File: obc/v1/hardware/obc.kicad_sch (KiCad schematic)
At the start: 41 parts, among them J4 USB_C_Receptacle_USB2.0_16P, U10 LM66100DCK, U11 LM66100DCK, U12 USBLC6-2P6, U9 AMS1117-3.3

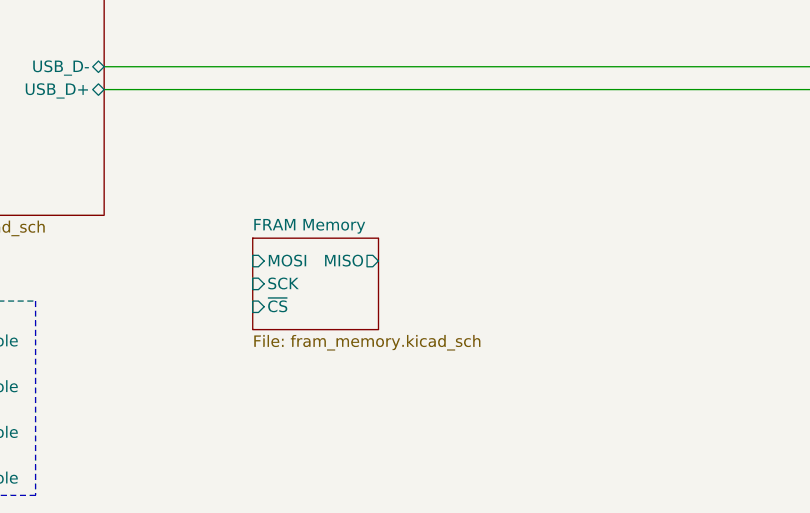
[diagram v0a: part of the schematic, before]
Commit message: fixes
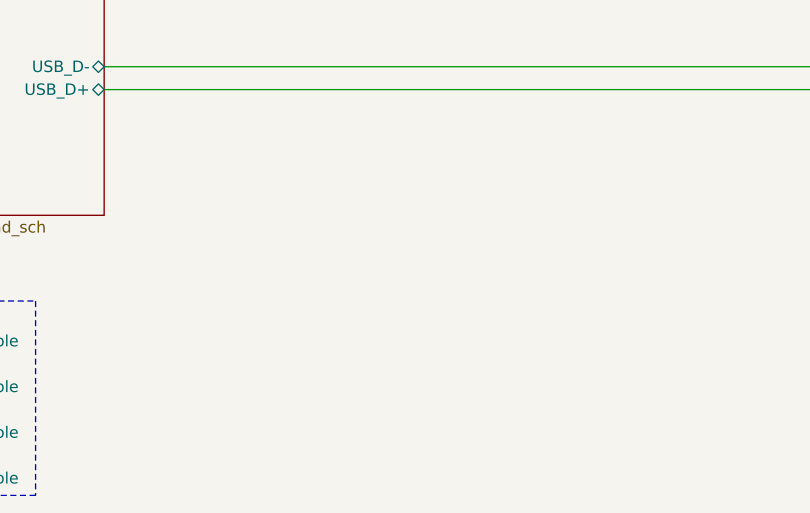
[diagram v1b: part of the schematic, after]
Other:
- removed sheet FRAM Memory
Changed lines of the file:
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@@
-	)
-	(sheet
-		(at 63.5 151.13)
-		(size 13.97 10.16)
-		(exclude_from_sim no)
-		(in_bom yes)
-		(on_board yes)
-		(dnp no)
-		(fields_autoplaced yes)
-		(stroke
-			(width 0.1524)
-			(type solid)
-		)
-		(fill
-			(color 0 0 0 0)
-		)
-		(property "Sheetname" "FRAM Memory"
-			(at 63.5 150.4184 0)
-			(show_name no)
-			(do_not_autoplace no)
-			(effects
-				(font
-					(size 1.27 1.27)
-				)
-				(justify left bottom)
-			)
-		)
-		(property "Sheetfile" "fram_memory.kicad_sch"
-			(at 63.5 161.8746 0)
-			(show_name no)
-			(do_not_autoplace no)
-			(effects
-				(font
-					(size 1.27 1.27)
-				)
-				(justify left top)
-			)
-		)
-		(pin "MOSI" input
-			(at 63.5 153.67 180)
-			(effects
-				(font
-					(size 1.27 1.27)
-				)
-				(justify left)
-			)
-		)
-		(pin "SCK" input
-			(at 63.5 156.21 180)
-			(effects
-				(font
-					(size 1.27 1.27)
-				)
-				(justify left)
-			)
-		)
-		(pin "~{CS}" input
-			(at 63.5 158.75 180)
-			(effects
-				(font
-					(size 1.27 1.27)
-				)
-				(justify left)
-			)
-		)
-		(pin "MISO" output
-			(at 77.47 153.67 0)
-			(effects
-				(font
-					(size 1.27 1.27)
-				)
-				(justify right)
-			)
-		)
-		(instances
-			(project "obc"
-				(path "/ba4f88ff-24aa-49a3-8871-8c7e48b371c5"
-					(page "10")
-				)
-			)
-		)
 	)
 	(sheet
